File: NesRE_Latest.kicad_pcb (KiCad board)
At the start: 2 copper layers, 195.6 x 120 mm, 32 parts

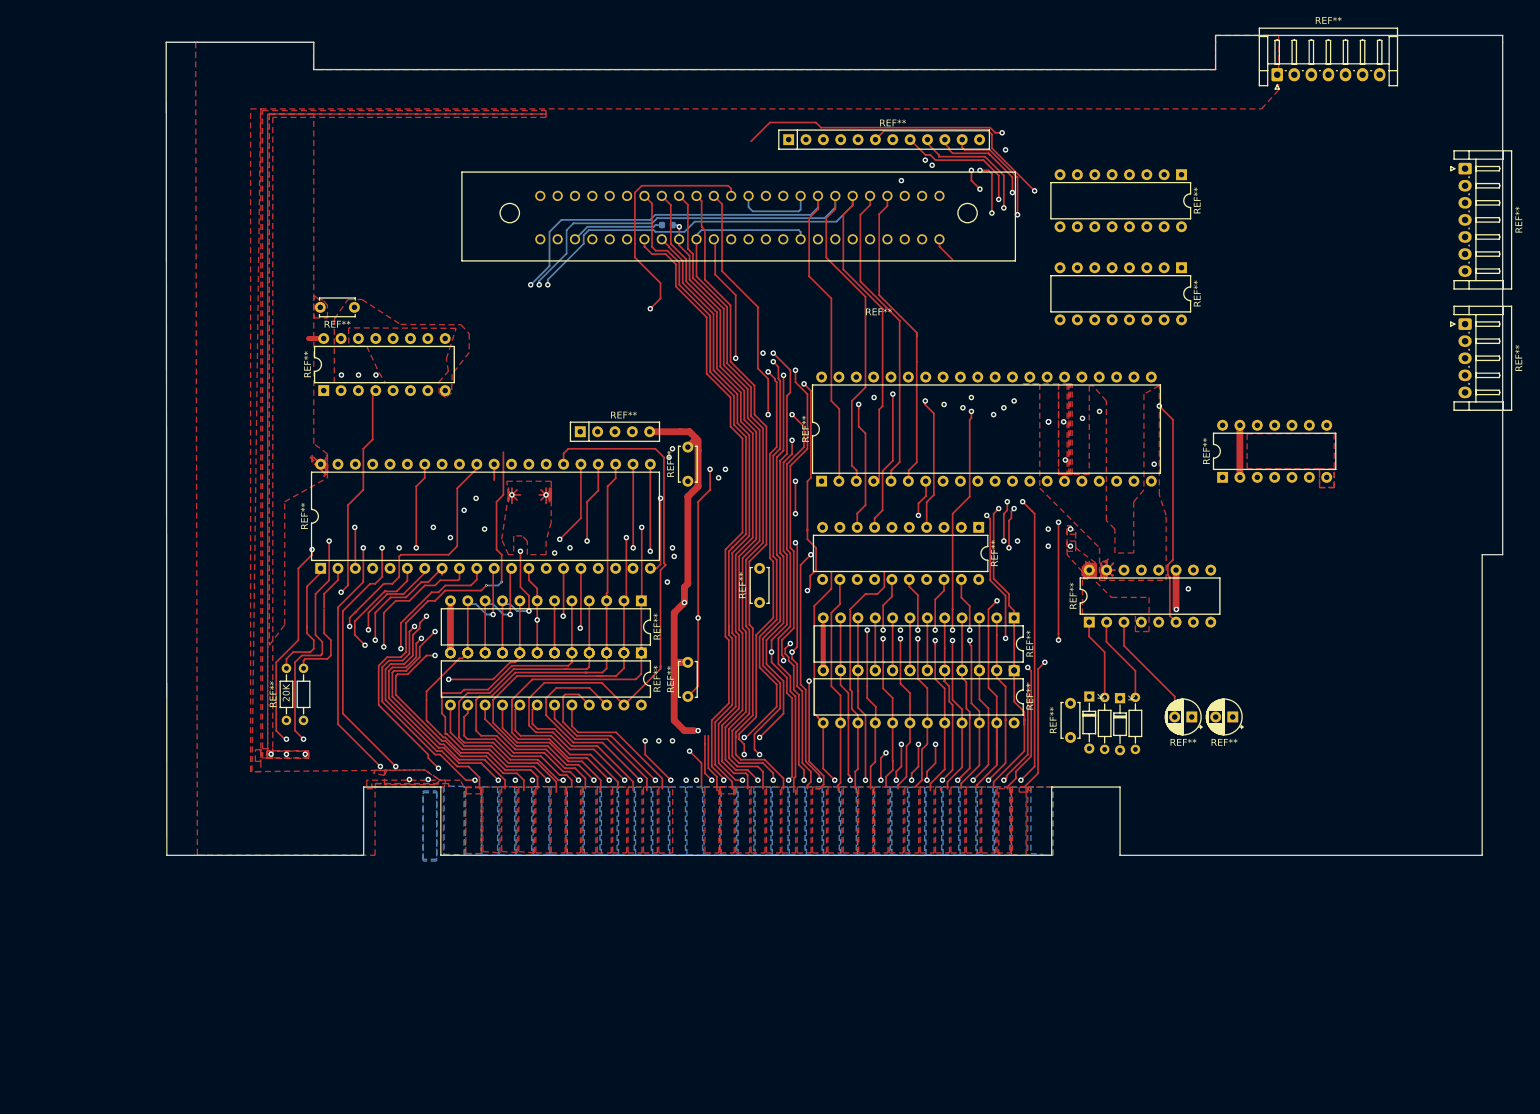
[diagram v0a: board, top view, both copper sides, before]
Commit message: Add files via upload
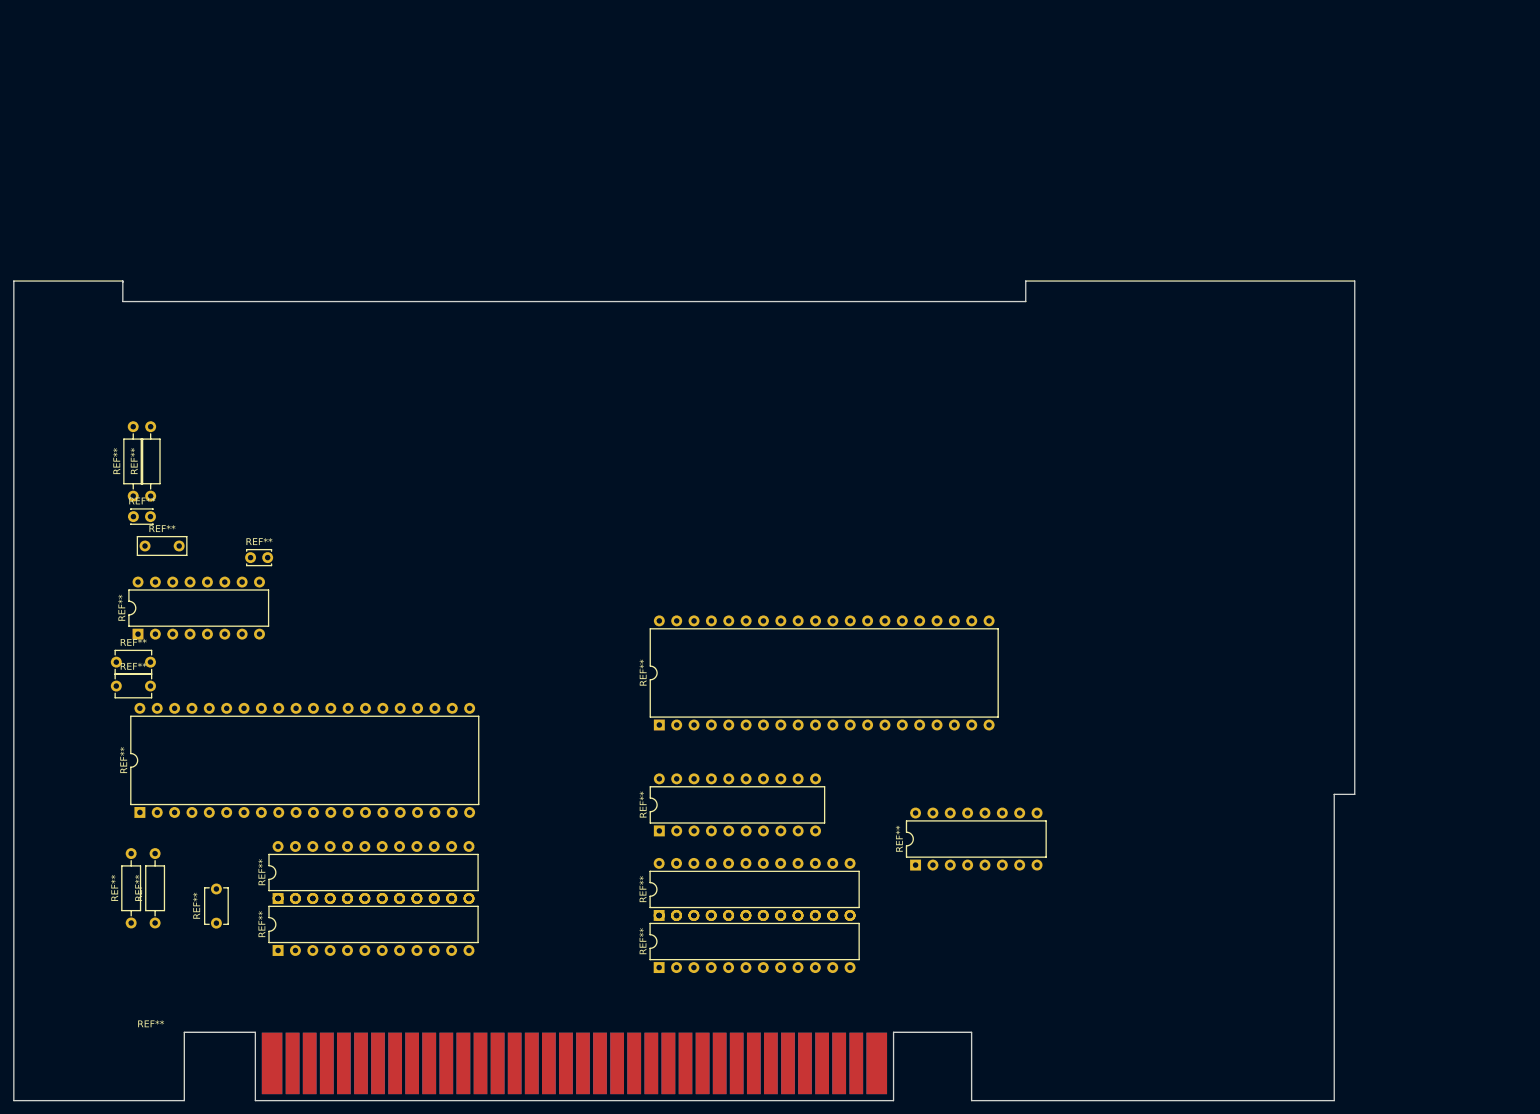
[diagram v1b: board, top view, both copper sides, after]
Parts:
- removed  : , Diode_THT:D_DO-34_SOD68_P7.62mm_Horizontal (x2)
- removed  : , Resistor_THT:R_Axial_DIN0204_L3.6mm_D1.6mm_P7.62mm_Horizontal (x2)
- removed 20K: , Resistor_THT:R_Axial_DIN0204_L3.6mm_D1.6mm_P7.62mm_Horizontal
- removed the REF** at (107.8, 69.8)
- removed the REF** at (62.0, 81.8)
- removed the REF** at (95.0, 100.0)
- removed the REF** at (110.8, 107.2)
- removed the REF** at (110.8, 138.8)
- removed the REF** at (121.2, 125.0)
- removed the REF** at (52.0, 142.2)
- removed the REF** at (125.5, 57.2)
- removed the REF** at (138.7, 82.0)
- removed the REF** at (103.9, 132.4)
- removed the REF** at (103.9, 124.8)
- removed the REF** at (190.5, 141.8)
- removed the REF** at (158.5, 127.2)
- removed the REF** at (189.0, 106.7)
- removed the REF** at (183.0, 76.0)
- removed the REF** at (183.0, 62.4)
- removed the REF** at (169.5, 127.9)
- removed the REF** at (158.5, 135.0)
- removed the REF** at (57.5, 94.0)
- removed the REF** at (184.5, 141.8)
- removed the REF** at (166.8, 144.8)
- removed the REF** at (224.5, 84.2)
- removed the REF** at (224.5, 61.5)
- removed the REF** at (197.0, 47.8)
- removed the REF** at (130.3, 107.2)
- removed the REF** at (57.0, 120.0)
- added REF**: DIP-16_W7.62mm, Package_DIP:DIP-16_W7.62mm, F.Cu at (144.1, 163.4)
- added REF**: C_Disc_D5.1mm_W3.2mm_P5.00mm, Capacitor_THT:C_Disc_D5.1mm_W3.2mm_P5.00mm, F.Cu at (27.1, 137.2)
- added REF**: DIP-16_W7.62mm, Package_DIP:DIP-16_W7.62mm, F.Cu at (30.3, 129.6)
- added REF**: DIP-40_W15.24mm, Package_DIP:DIP-40_W15.24mm, F.Cu at (30.6, 155.7)
- added REF**: DIP-24_W7.62mm, Package_DIP:DIP-24_W7.62mm, F.Cu at (106.5, 170.8)
- added REF**: DIP-24_W7.62mm, Package_DIP:DIP-24_W7.62mm, F.Cu at (106.5, 178.4)
- added REF**: DIP-24_W7.62mm, Package_DIP:DIP-24_W7.62mm, F.Cu at (50.8, 168.3)
- added REF**: DIP-24_W7.62mm, Package_DIP:DIP-24_W7.62mm, F.Cu at (50.8, 175.9)
- added REF**: C_Disc_D5.1mm_W3.2mm_P5.00mm, Capacitor_THT:C_Disc_D5.1mm_W3.2mm_P5.00mm, F.Cu at (41.8, 171.9)
- added REF**: R_Axial_DIN0207_L6.3mm_D2.5mm_P10.16mm_Horizontal, Resistor_THT:R_Axial_DIN0207_L6.3mm_D2.5mm_P10.16mm_Horizontal, F.Cu at (32.8, 171.9)
- added REF**: R_Axial_DIN0207_L6.3mm_D2.5mm_P10.16mm_Horizontal, Resistor_THT:R_Axial_DIN0207_L6.3mm_D2.5mm_P10.16mm_Horizontal, F.Cu at (29.3, 171.9)
- added REF**: NES_Edge_Connector, NESReSize:NES_Edge_Connector, F.Cu at (32.1, 186.2)
- added REF**: DIP-40_W15.24mm, Package_DIP:DIP-40_W15.24mm, F.Cu at (106.6, 142.9)
- added REF**: R_Axial_DIN0207_L6.3mm_D2.5mm_P10.16mm_Horizontal, Resistor_THT:R_Axial_DIN0207_L6.3mm_D2.5mm_P10.16mm_Horizontal, F.Cu at (32.1, 109.4)
- added REF**: R_Axial_DIN0207_L6.3mm_D2.5mm_P10.16mm_Horizontal, Resistor_THT:R_Axial_DIN0207_L6.3mm_D2.5mm_P10.16mm_Horizontal, F.Cu at (29.6, 109.4)
- added REF**: C_Disc_D3.0mm_W2.0mm_P2.50mm, Capacitor_THT:C_Disc_D3.0mm_W2.0mm_P2.50mm, F.Cu at (29.6, 112.4)
- added REF**: C_Disc_D7.0mm_W2.5mm_P5.00mm, Capacitor_THT:C_Disc_D7.0mm_W2.5mm_P5.00mm, F.Cu at (31.3, 116.7)
- added REF**: C_Disc_D3.4mm_W2.1mm_P2.50mm, Capacitor_THT:C_Disc_D3.4mm_W2.1mm_P2.50mm, F.Cu at (46.8, 118.4)
- added REF**: C_Disc_D5.1mm_W3.2mm_P5.00mm, Capacitor_THT:C_Disc_D5.1mm_W3.2mm_P5.00mm, F.Cu at (27.1, 133.7)
- moved REF** 64.5 mm to (106.6, 158.4), turned to 90 degrees
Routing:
- net (no net): track 4522.7 -> 0.00 mm, vias 210 -> 0
- removed copper zone on B.Cu, net (none)
- removed copper zone on F.Cu, net (none)
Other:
- board size 195.6 x 120 mm -> 196.2 x 120 mm
- rule pad_to_mask_clearance: 0 -> 0.051
- board text removed: "www.Github.com/Redherring32"
